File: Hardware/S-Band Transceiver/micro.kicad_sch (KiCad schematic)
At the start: 3 parts, among them J2 AVR-UPDI-6, U11 AVR128DA48x-xPT, U12 ADS1118IDGS

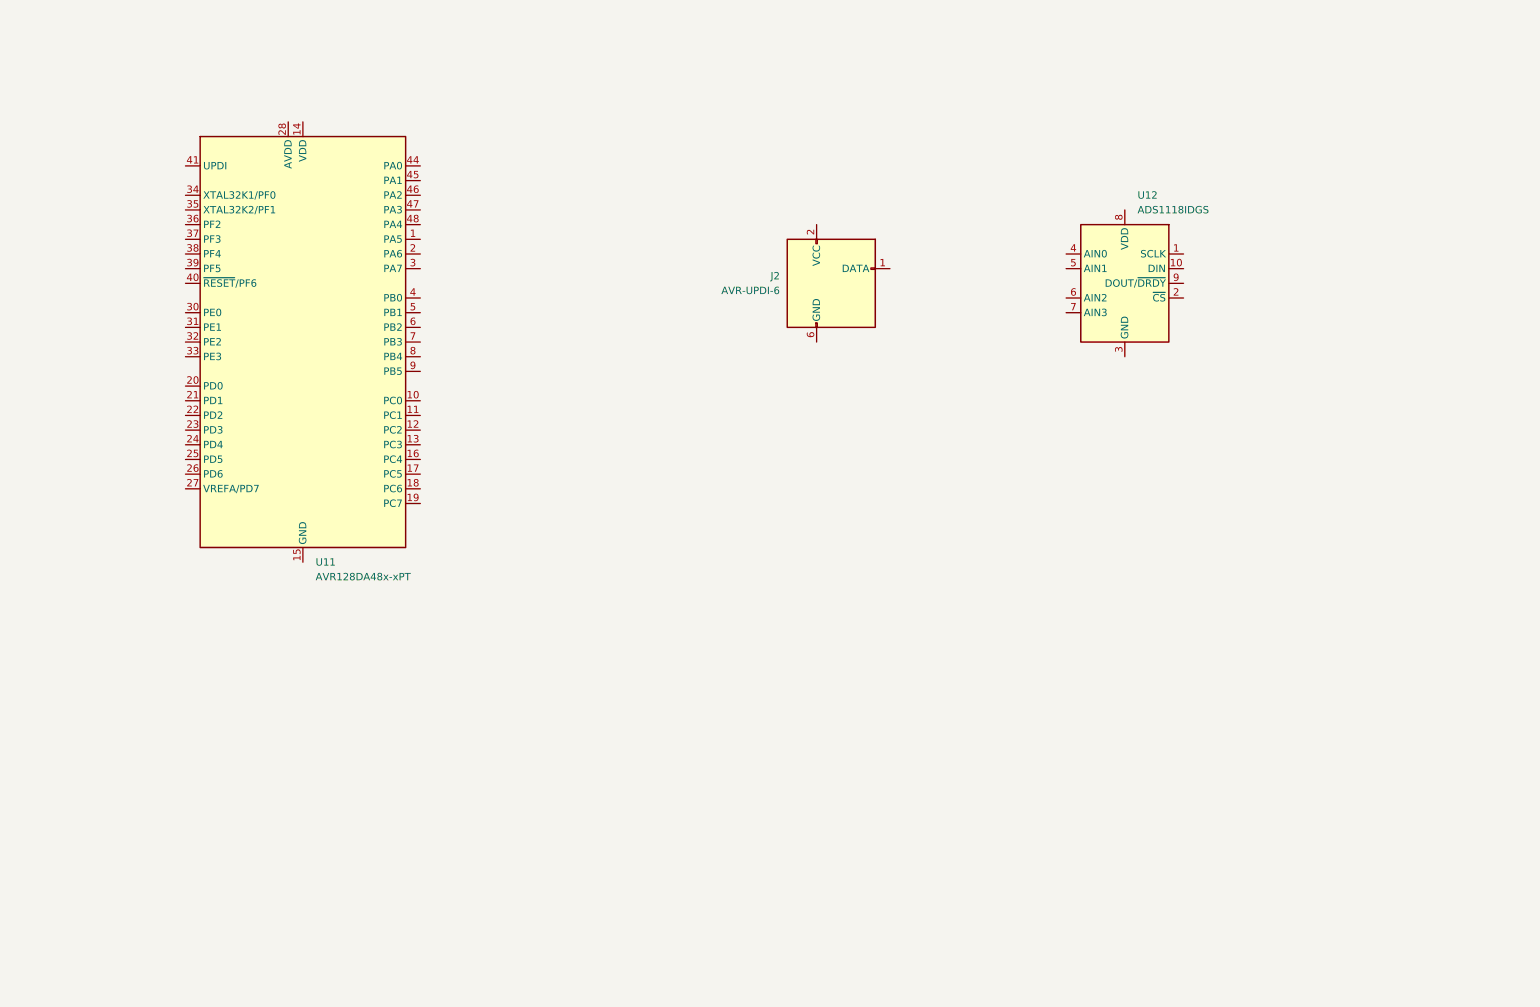
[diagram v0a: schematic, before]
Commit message: Updates to schematic
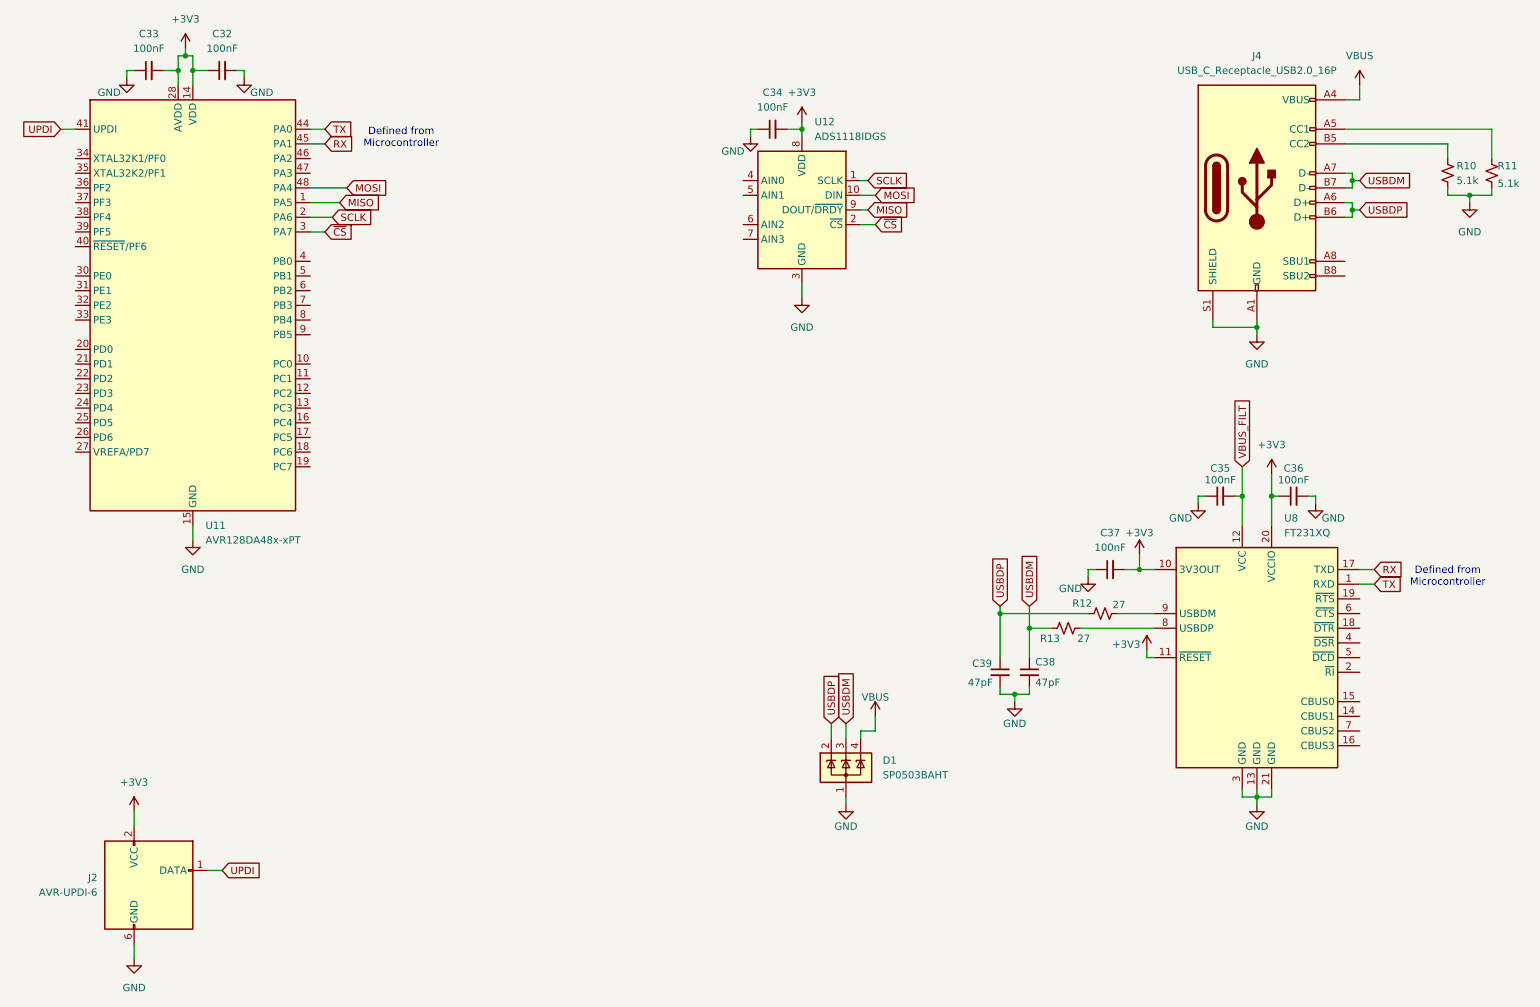
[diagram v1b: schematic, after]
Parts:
- added C32, C33, C34, C35, C36, C37: 100nF, symbol Device:C_Small
- added C38, C39: 47pF, symbol Device:C_Small
- added D1: SP0503BAHT, Package_TO_SOT_SMD:SOT-143, symbol Power_Protection:SP0503BAHT
- added J4: USB_C_Receptacle_USB2.0_16P, symbol Connector:USB_C_Receptacle_USB2.0_16P
- added R10, R11: 5.1k, symbol Device:R_Small_US
- added R12, R13: 27, symbol Device:R_Small_US
- added U8: FT231XQ, Package_DFN_QFN:QFN-20-1EP_4x4mm_P0.5mm_EP2.5x2.5mm, symbol Interface_USB:FT231XQ
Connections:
- net SCLK: now reaches U12.1 (SCLK)
- net SCLK: now also U11.2 (PA6)
- net MOSI: now reaches U12.10 (DIN)
- net MOSI: now also U11.48 (PA4)
- net ~{CS}: now reaches U12.2 (~{CS})
- net ~{CS}: now also U11.3 (PA7)
- net GND: now reaches U12.3 (GND)
- net GND: now also J2.6 (GND), U11.15 (GND), U11.29 (GND), U11.43 (GND), C32.2, C33.1, C34.1, C35.1, C36.2, C37.1, C38.2, C39.2, D1.1 (A), J4.A1 (GND), J4.A12 (GND), J4.B1 (GND), J4.B12 (GND), J4.S1 (SHIELD), R10.2, R11.2, U8.13 (GND), U8.21 (GND), U8.3 (GND)
- net +3V3: now reaches U12.8 (VDD)
- net +3V3: now also J2.2 (VCC), U11.14 (VDD), U11.28 (AVDD), U11.42 (VDD), C32.1, C33.2, C34.2, C36.1, C37.2, U8.10 (3V3OUT), U8.11 (~{RESET}), U8.20 (VCCIO)
- net MISO: now reaches U12.9 (DOUT/~{DRDY})
- net MISO: now also U11.1 (PA5)
- net UPDI: now reaches U11.41 (UPDI)
- net UPDI: now also J2.1 (DATA)
- net TX: now reaches U11.44 (PA0)
- net TX: now also U8.1 (RXD)
- net RX: now reaches U11.45 (PA1)
- net RX: now also U8.17 (TXD)
- new net: J4.A5 (CC1), R11.1
- new net: R13.2, U8.8 (USBDP)
- new net: J4.B5 (CC2), R10.1
- new net: R12.2, U8.9 (USBDM)
- new net USBDM: C38.1, D1.3 (K), J4.A7 (D-), J4.B7 (D-), R13.1
- new net USBDP: C39.1, D1.2 (K), J4.A6 (D+), J4.B6 (D+), R12.1
- new net VBUS: D1.4 (K), J4.A4 (VBUS), J4.A9 (VBUS), J4.B4 (VBUS), J4.B9 (VBUS)
- new net VBUS_FILT: C35.2, U8.12 (VCC)
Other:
- note added: "Defined from Microcontroller"
- moved on the sheet: J2, U11, U12
